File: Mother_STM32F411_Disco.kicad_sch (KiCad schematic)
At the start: 15 parts

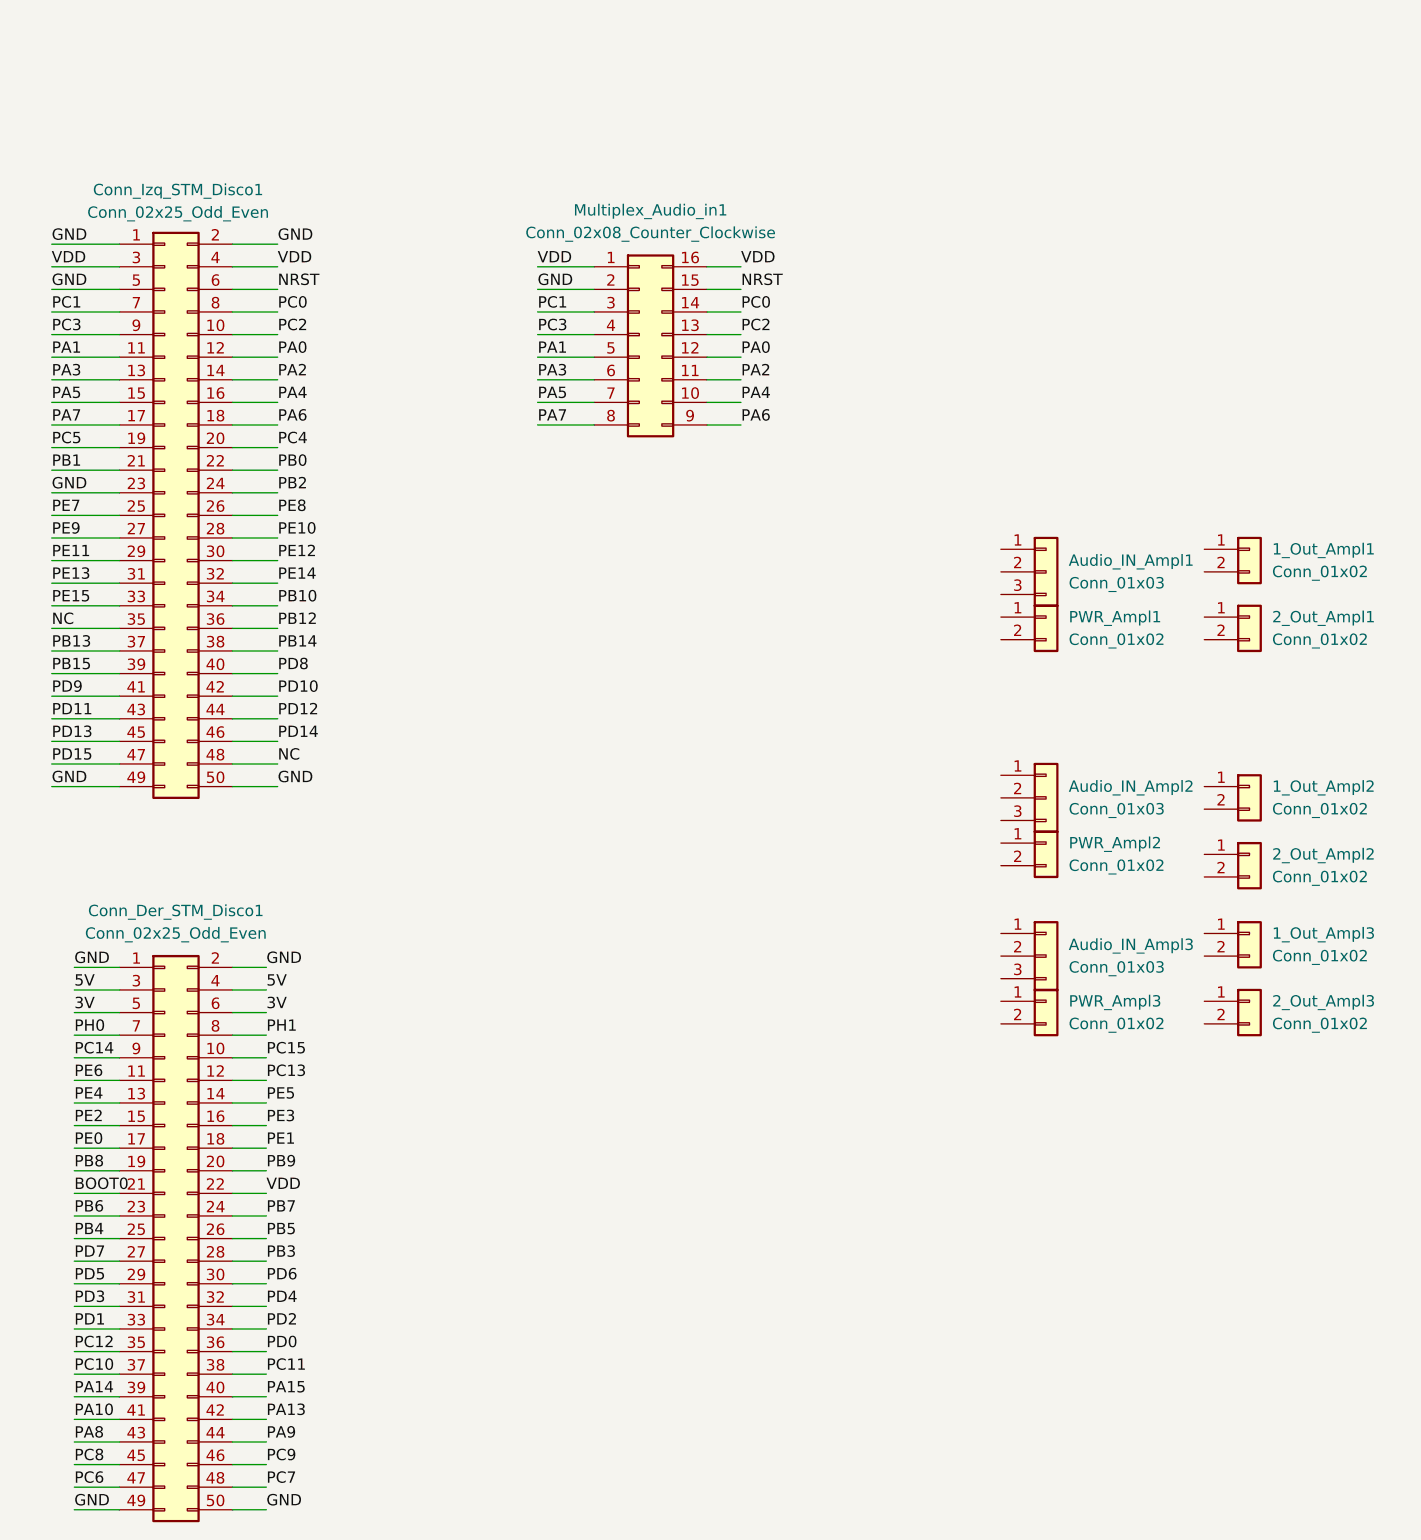
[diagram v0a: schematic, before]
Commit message: Huellas y netlist
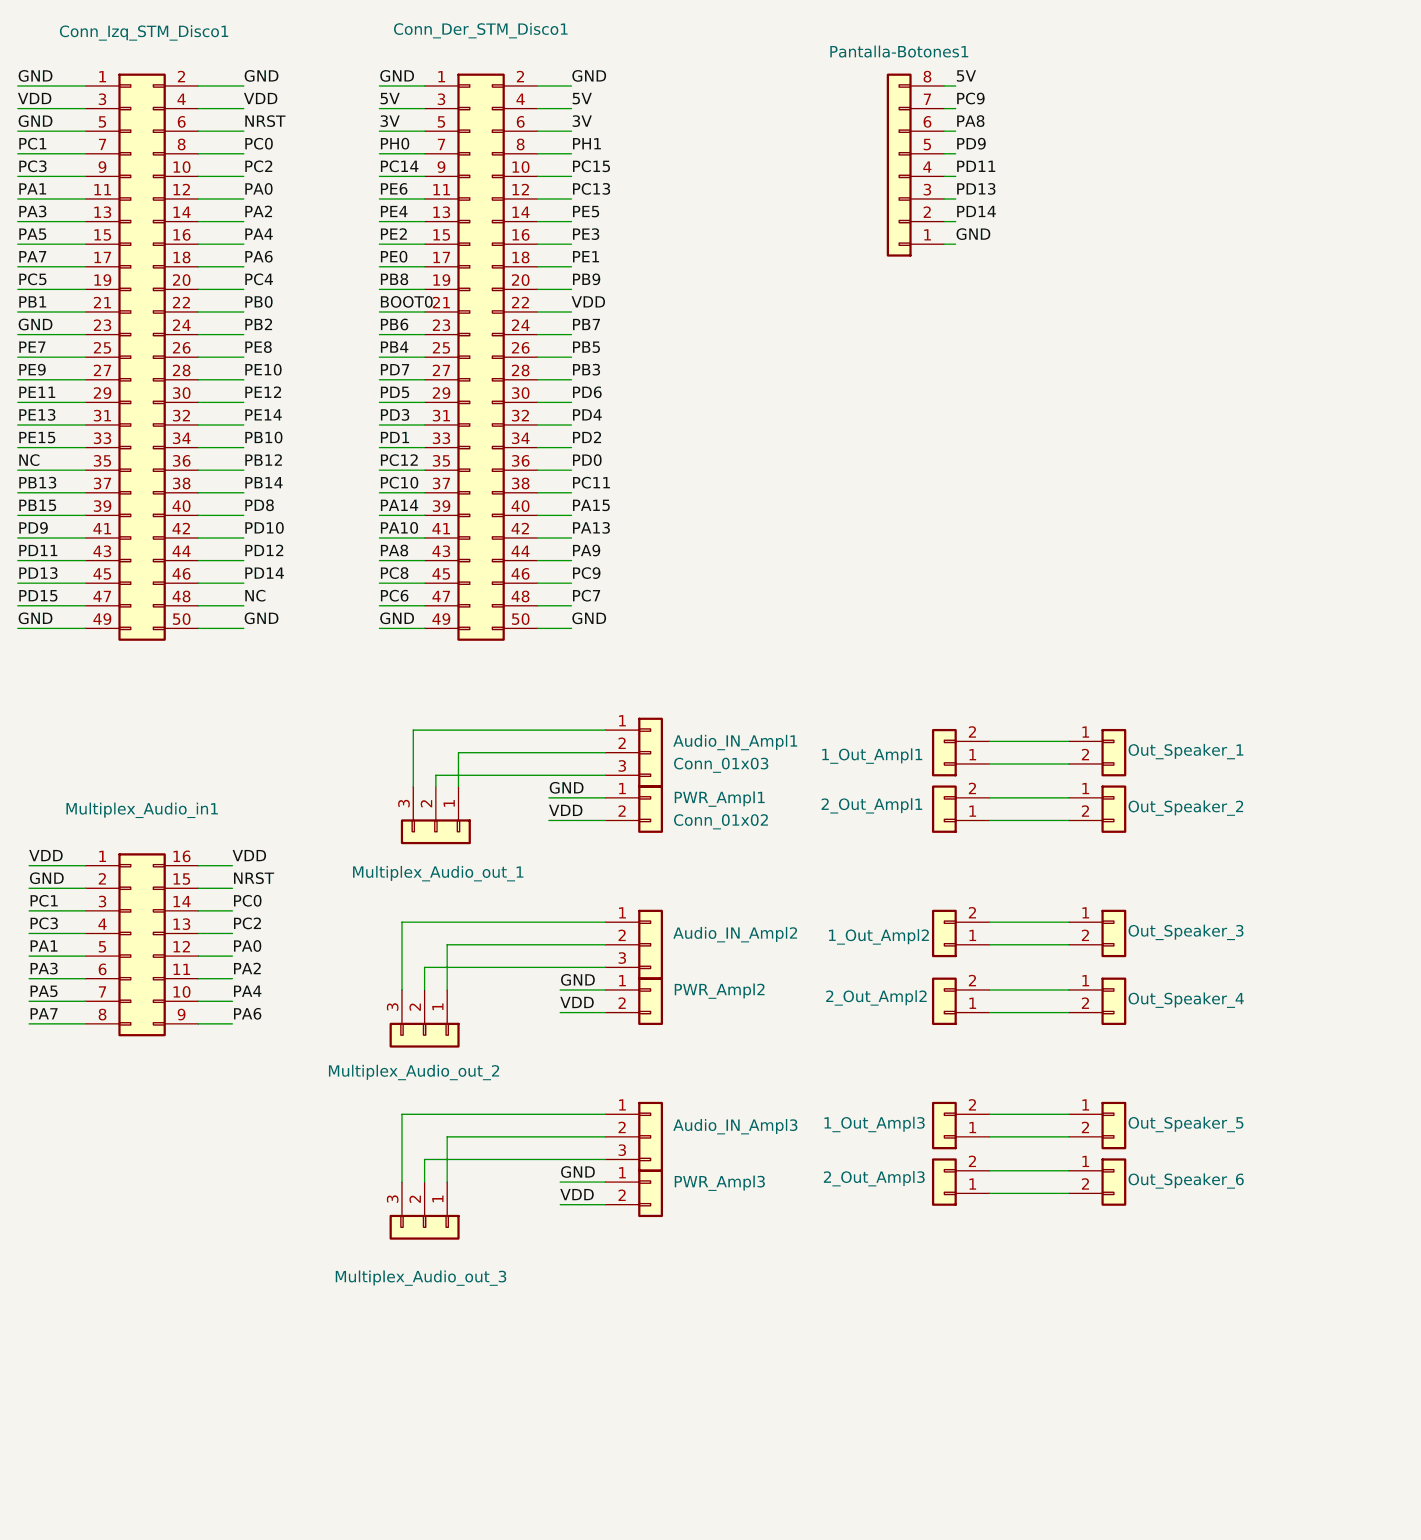
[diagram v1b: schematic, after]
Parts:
- added Multiplex_Audio_out_1, Multiplex_Audio_out_2, Multiplex_Audio_out_3: Conn_01x03, Connector_PinSocket_2.54mm:PinSocket_1x03_P2.54mm_Vertical, symbol Connector_Generic:Conn_01x03
- added Out_Speaker_1, Out_Speaker_2, Out_Speaker_3, Out_Speaker_4, Out_Speaker_5, Out_Speaker_6: Conn_01x02, Connector_PinHeader_2.54mm:PinHeader_1x02_P2.54mm_Horizontal, symbol Connector_Generic:Conn_01x02
- added Pantalla-Botones1: Conn_01x08, Connector_PinSocket_2.54mm:PinSocket_1x08_P2.54mm_Vertical, symbol Connector_Generic:Conn_01x08
- 1_Out_Ampl1, 1_Out_Ampl2, 1_Out_Ampl3, 2_Out_Ampl1, 2_Out_Ampl2, 2_Out_Ampl3, PWR_Ampl1, PWR_Ampl2, PWR_Ampl3: footprint (none) -> Connector_PinSocket_2.54mm:PinSocket_1x02_P2.54mm_Vertical
- Audio_IN_Ampl1, Audio_IN_Ampl2, Audio_IN_Ampl3: footprint (none) -> Connector_PinSocket_2.54mm:PinSocket_1x03_P2.54mm_Vertical
- Multiplex_Audio_in1: footprint (none) -> Connector_PinSocket_2.54mm:PinSocket_2x08_P2.54mm_Vertical
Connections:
- net 5V: now also Pantalla-Botones1.8 (Pin_8)
- net GND: now also PWR_Ampl1.1 (Pin_1), PWR_Ampl2.1 (Pin_1), PWR_Ampl3.1 (Pin_1), Pantalla-Botones1.1 (Pin_1)
- net PA8: now also Pantalla-Botones1.6 (Pin_6)
- net PC9: now also Pantalla-Botones1.7 (Pin_7)
- net PD11: now also Pantalla-Botones1.4 (Pin_4)
- net PD13: now also Pantalla-Botones1.3 (Pin_3)
- net PD14: now also Pantalla-Botones1.2 (Pin_2)
- net PD9: now also Pantalla-Botones1.5 (Pin_5)
- net VDD: now also PWR_Ampl1.2 (Pin_2), PWR_Ampl2.2 (Pin_2), PWR_Ampl3.2 (Pin_2)
- net at 2_Out_Ampl2.1 (Pin_1): now also Out_Speaker_4.2 (Pin_2)
- net at 2_Out_Ampl2.2 (Pin_2): now also Out_Speaker_4.1 (Pin_1)
- net at 1_Out_Ampl2.1 (Pin_1): now also Out_Speaker_3.2 (Pin_2)
- net at 1_Out_Ampl2.2 (Pin_2): now also Out_Speaker_3.1 (Pin_1)
- net at 1_Out_Ampl1.1 (Pin_1): now also Out_Speaker_1.2 (Pin_2)
- net at 1_Out_Ampl1.2 (Pin_2): now also Out_Speaker_1.1 (Pin_1)
- net at 2_Out_Ampl1.1 (Pin_1): now also Out_Speaker_2.2 (Pin_2)
- net at 2_Out_Ampl1.2 (Pin_2): now also Out_Speaker_2.1 (Pin_1)
- net at Audio_IN_Ampl1.1 (Pin_1): now also Multiplex_Audio_out_1.3 (Pin_3)
- net at Audio_IN_Ampl1.2 (Pin_2): now also Multiplex_Audio_out_1.1 (Pin_1)
- net at Audio_IN_Ampl1.3 (Pin_3): now also Multiplex_Audio_out_1.2 (Pin_2)
- net at Audio_IN_Ampl3.1 (Pin_1): now also Multiplex_Audio_out_3.3 (Pin_3)
- net at Audio_IN_Ampl3.2 (Pin_2): now also Multiplex_Audio_out_3.1 (Pin_1)
- net at Audio_IN_Ampl3.3 (Pin_3): now also Multiplex_Audio_out_3.2 (Pin_2)
- net at 1_Out_Ampl3.1 (Pin_1): now also Out_Speaker_5.2 (Pin_2)
- net at 1_Out_Ampl3.2 (Pin_2): now also Out_Speaker_5.1 (Pin_1)
- net at Audio_IN_Ampl2.1 (Pin_1): now also Multiplex_Audio_out_2.3 (Pin_3)
- net at Audio_IN_Ampl2.2 (Pin_2): now also Multiplex_Audio_out_2.1 (Pin_1)
- net at Audio_IN_Ampl2.3 (Pin_3): now also Multiplex_Audio_out_2.2 (Pin_2)
- net at 2_Out_Ampl3.1 (Pin_1): now also Out_Speaker_6.2 (Pin_2)
- net at 2_Out_Ampl3.2 (Pin_2): now also Out_Speaker_6.1 (Pin_1)
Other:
- moved on the sheet: 1_Out_Ampl1, 1_Out_Ampl2, 1_Out_Ampl3, 2_Out_Ampl1, 2_Out_Ampl2, 2_Out_Ampl3, Audio_IN_Ampl1, Audio_IN_Ampl2, Audio_IN_Ampl3, Conn_Der_STM_Disco1, Conn_Izq_STM_Disco1, Multiplex_Audio_in1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
